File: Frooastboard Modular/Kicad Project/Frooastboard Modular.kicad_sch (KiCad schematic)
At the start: 40 parts, among them J1 Conn_01x16, J2 Conn_01x06, J3 Conn_01x06, J4 Conn_01x10, J5 Conn_01x12, J6 SW Interface, J7 Conn_01x04, U1 IS31FL3733-QF, U2 RP2040, U3 W25Q32JVZP, U4 LM317L_SOT-89, Y1 12MHz

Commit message: basic left side
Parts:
- R10: footprint Resistor_SMD:R_0402_1005Metric -> Resistor_SMD:R_0805_2012Metric
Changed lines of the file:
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@@
       (effects (font (size 1.27 1.27)))
     )
-    (property "Footprint" "Resistor_SMD:R_0402_1005Metric" (at 182.88 39.37 0)
+    (property "Footprint" "Resistor_SMD:R_0805_2012Metric" (at 182.88 39.37 0)
       (effects (font (size 1.27 1.27)) hide)
     )

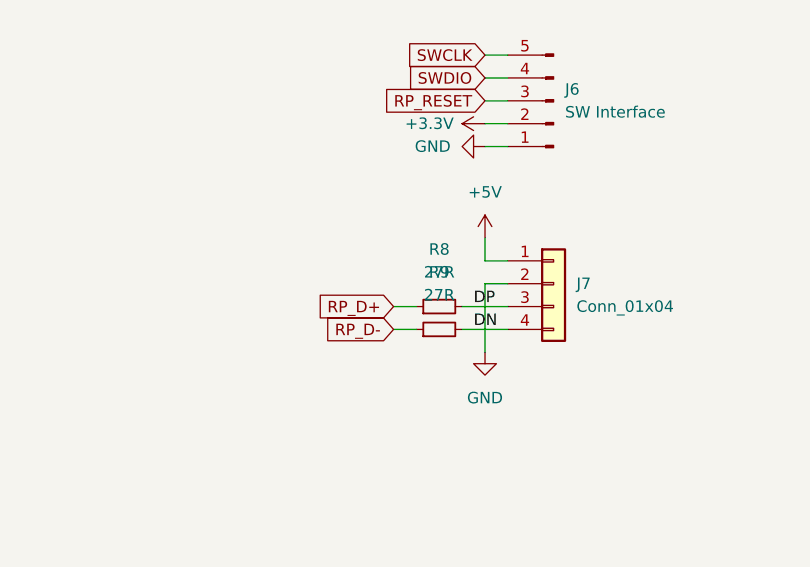
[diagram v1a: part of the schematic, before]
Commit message: backup before differential
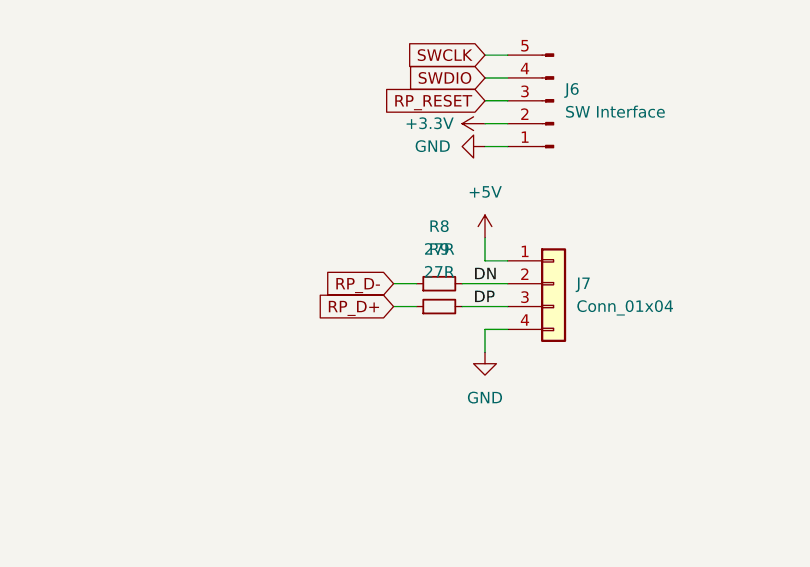
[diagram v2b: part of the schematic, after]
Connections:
- net DN: now also J7.2 (Pin_2), R8.2; no longer J7.4 (Pin_4), R9.2
- net DP: now also R9.2; no longer R8.2
- net GND: now also J7.4 (Pin_4); no longer J7.2 (Pin_2)
- net RP_D+: now also R9.1; no longer R8.1
- net RP_D-: now also R8.1; no longer R9.1
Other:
- moved on the sheet: R8, R9
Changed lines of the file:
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@@
     (stroke (width 0) (type default))
   )
+  (wire (pts (xy 186.69 135.89) (xy 186.69 138.43))
+    (stroke (width 0) (type default))
+  )
   (wire (pts (xy 68.58 267.97) (xy 66.04 267.97))
     (stroke (width 0) (type default))
@@
     (stroke (width 0) (type default))
   )
-  (wire (pts (xy 189.23 130.81) (xy 186.69 130.81))
-    (stroke (width 0) (type default))
-  )
   (wire (pts (xy 83.82 217.17) (xy 86.36 217.17))
     (stroke (width 0) (type default))
@@
     (stroke (width 0) (type default))
   )
-  (wire (pts (xy 184.15 133.35) (xy 189.23 133.35))
+  (wire (pts (xy 184.15 130.81) (xy 189.23 130.81))
     (stroke (width 0) (type default))
   )
@@
     (stroke (width 0) (type default))
   )
-  (wire (pts (xy 184.15 135.89) (xy 189.23 135.89))
+  (wire (pts (xy 184.15 133.35) (xy 189.23 133.35))
     (stroke (width 0) (type default))
   )
@@
     (stroke (width 0) (type default))
   )
-  (wire (pts (xy 176.53 135.89) (xy 179.07 135.89))
+  (wire (pts (xy 176.53 133.35) (xy 179.07 133.35))
     (stroke (width 0) (type default))
   )
@@
     (stroke (width 0) (type default))
   )
-  (wire (pts (xy 186.69 130.81) (xy 186.69 138.43))
-    (stroke (width 0) (type default))
-  )
   (wire (pts (xy 46.99 60.96) (xy 49.53 60.96))
     (stroke (width 0) (type default))
@@
     (stroke (width 0) (type default))
   )
-  (wire (pts (xy 176.53 133.35) (xy 179.07 133.35))
+  (wire (pts (xy 176.53 130.81) (xy 179.07 130.81))
     (stroke (width 0) (type default))
   )
@@
     (stroke (width 0) (type default))
   )
+  (wire (pts (xy 189.23 135.89) (xy 186.69 135.89))
+    (stroke (width 0) (type default))
+  )
   (wire (pts (xy 46.99 26.67) (xy 62.23 26.67))
     (stroke (width 0) (type default))
@@
     (stroke (width 0) (type default))
   )
-  (label "DP" (at 185.42 133.35 0) (fields_autoplaced)
+  (label "DN" (at 185.42 130.81 0) (fields_autoplaced)
     (effects (font (size 1.27 1.27)) (justify left bottom))
   )
-  (label "DN" (at 185.42 135.89 0) (fields_autoplaced)
+  (label "DP" (at 185.42 133.35 0) (fields_autoplaced)
     (effects (font (size 1.27 1.27)) (justify left bottom))
   )
@@
     )
   )
-  (global_label "RP_D-" (shape input) (at 176.53 135.89 180) (fields_autoplaced)
+  (global_label "RP_D-" (shape input) (at 176.53 130.81 180) (fields_autoplaced)
     (effects (font (size 1.27 1.27)) (justify right))
-    (property "Intersheetrefs" "${INTERSHEET_REFS}" (at 167.7669 135.8106 0)
+    (property "Intersheetrefs" "${INTERSHEET_REFS}" (at 167.7669 130.7306 0)
       (effects (font (size 1.27 1.27)) (justify right) hide)
     )
@@
     )
   )
-  (symbol (lib_id "Device:R_Small") (at 181.61 133.35 90) (unit 1)
+  (symbol (lib_id "Device:R_Small") (at 181.61 130.81 90) (unit 1)
     (in_bom yes) (on_board yes) (dnp no) (fields_autoplaced)
-    (property "Reference" "R8" (at 181.61 127 90)
+    (property "Reference" "R8" (at 181.61 124.46 90)
       (effects (font (size 1.27 1.27)))
     )
-    (property "Value" "27R" (at 181.61 129.54 90)
+    (property "Value" "27R" (at 181.61 127 90)
       (effects (font (size 1.27 1.27)))
     )
-    (property "Footprint" "Resistor_SMD:R_0402_1005Metric" (at 181.61 133.35 0)
+    (property "Footprint" "Resistor_SMD:R_0402_1005Metric" (at 181.61 130.81 0)
       (effects (font (size 1.27 1.27)) hide)
     )
-    (property "Datasheet" "~" (at 181.61 133.35 0)
+    (property "Datasheet" "~" (at 181.61 130.81 0)
       (effects (font (size 1.27 1.27)) hide)
     )
@@
     )
   )
-  (symbol (lib_id "Device:R_Small") (at 181.61 135.89 90) (unit 1)
+  (symbol (lib_id "Device:R_Small") (at 181.61 133.35 90) (unit 1)
     (in_bom yes) (on_board yes) (dnp no) (fields_autoplaced)
-    (property "Reference" "R9" (at 181.61 129.54 90)
+    (property "Reference" "R9" (at 181.61 127 90)
       (effects (font (size 1.27 1.27)))
     )
-    (property "Value" "27R" (at 181.61 132.08 90)
+    (property "Value" "27R" (at 181.61 129.54 90)
       (effects (font (size 1.27 1.27)))
     )
-    (property "Footprint" "Resistor_SMD:R_0402_1005Metric" (at 181.61 135.89 0)
+    (property "Footprint" "Resistor_SMD:R_0402_1005Metric" (at 181.61 133.35 0)
       (effects (font (size 1.27 1.27)) hide)
     )
-    (property "Datasheet" "~" (at 181.61 135.89 0)
+    (property "Datasheet" "~" (at 181.61 133.35 0)
       (effects (font (size 1.27 1.27)) hide)
     )
